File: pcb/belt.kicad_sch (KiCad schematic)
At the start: 2 parts, among them U1 Raspberry-Pi-Pico, U2 Barometer-KP212K1409XTMA1

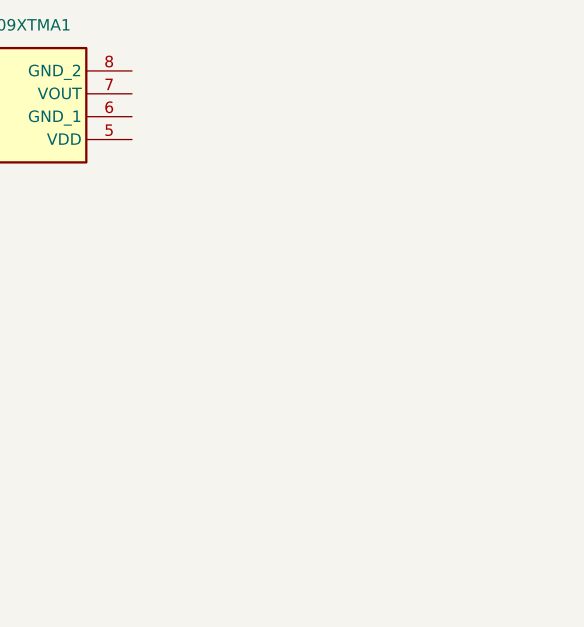
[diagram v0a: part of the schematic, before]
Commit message: added thermometer
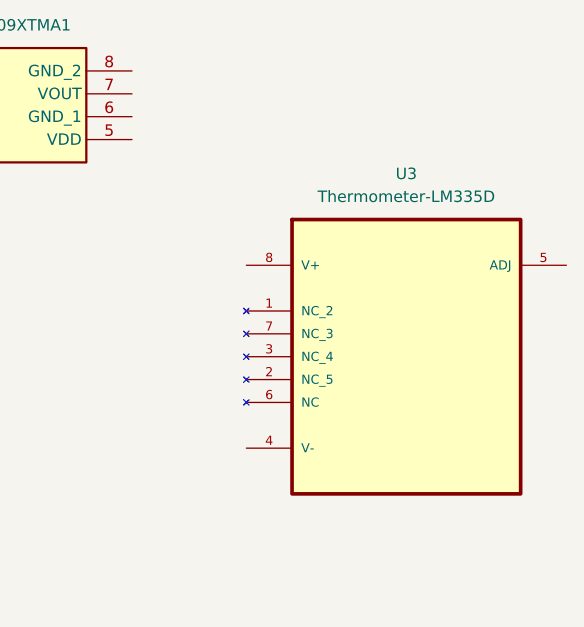
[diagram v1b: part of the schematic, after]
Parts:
- added U3: Thermometer-LM335D, BeltFootprints:Thermometer-LM335D, symbol Thermometer-LM335D:Thermometer-LM335D
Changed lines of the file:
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@@
   (title_block
     (title "Basic Electronics Learning Toolkit")
-    (date "2023-12-25")
+    (date "2023-12-26")
     (rev "0.1")
     (company "Rice Eclipse")
@@
         )
       )
+    )
+  )
+  (symbol (lib_id "Thermometer-LM335D:Thermometer-LM335D") (at 177.8 93.98 0) (unit 1)
+    (in_bom yes) (on_board yes) (dnp no) (fields_autoplaced)
+    (property "Reference" "U3" (at 177.8 73.66 0)
+      (effects (font (size 1.27 1.27)))
+    )
+    (property "Value" "Thermometer-LM335D" (at 177.8 76.2 0)
+      (effects (font (size 1.27 1.27)))
+    )
+    (property "Footprint" "BeltFootprints:Thermometer-LM335D" (at 177.8 116.84 0) (show_name)
+      (effects (font (size 1.27 1.27)) hide)
+    )
+    (property "Datasheet" "https://www.st.com/content/ccc/resource/technical/document/datasheet/04/fa/9d/16/39/87/44/8d/CD00000459.pdf/files/CD00000459.pdf/jcr:content/translations/en.CD00000459.pdf" (at 177.8 119.38 0) (show_name)
+      (effects (font (size 1.27 1.27)) hide)
+    )
+    (property "Manufacturer" "STMicroelectronics" (at 177.8 121.92 0) (show_name)
+      (effects (font (size 1.27 1.27)) hide)
+    )
+    (property "Part Number" "LM335D" (at 177.8 124.46 0) (show_name)
+      (effects (font (size 1.27 1.27)) hide)
+    )
+    (pin "1")
+    (pin "2")
+    (pin "3")
+    (pin "4")
+    (pin "5")
+    (pin "6")
+    (pin "7")
+    (pin "8")
+    (instances
+      (project "belt"
+        (path "/33e5c18d-f516-4ab7-aaea-c68685305111"
+          (reference "U3") (unit 1)
+        )
+      )

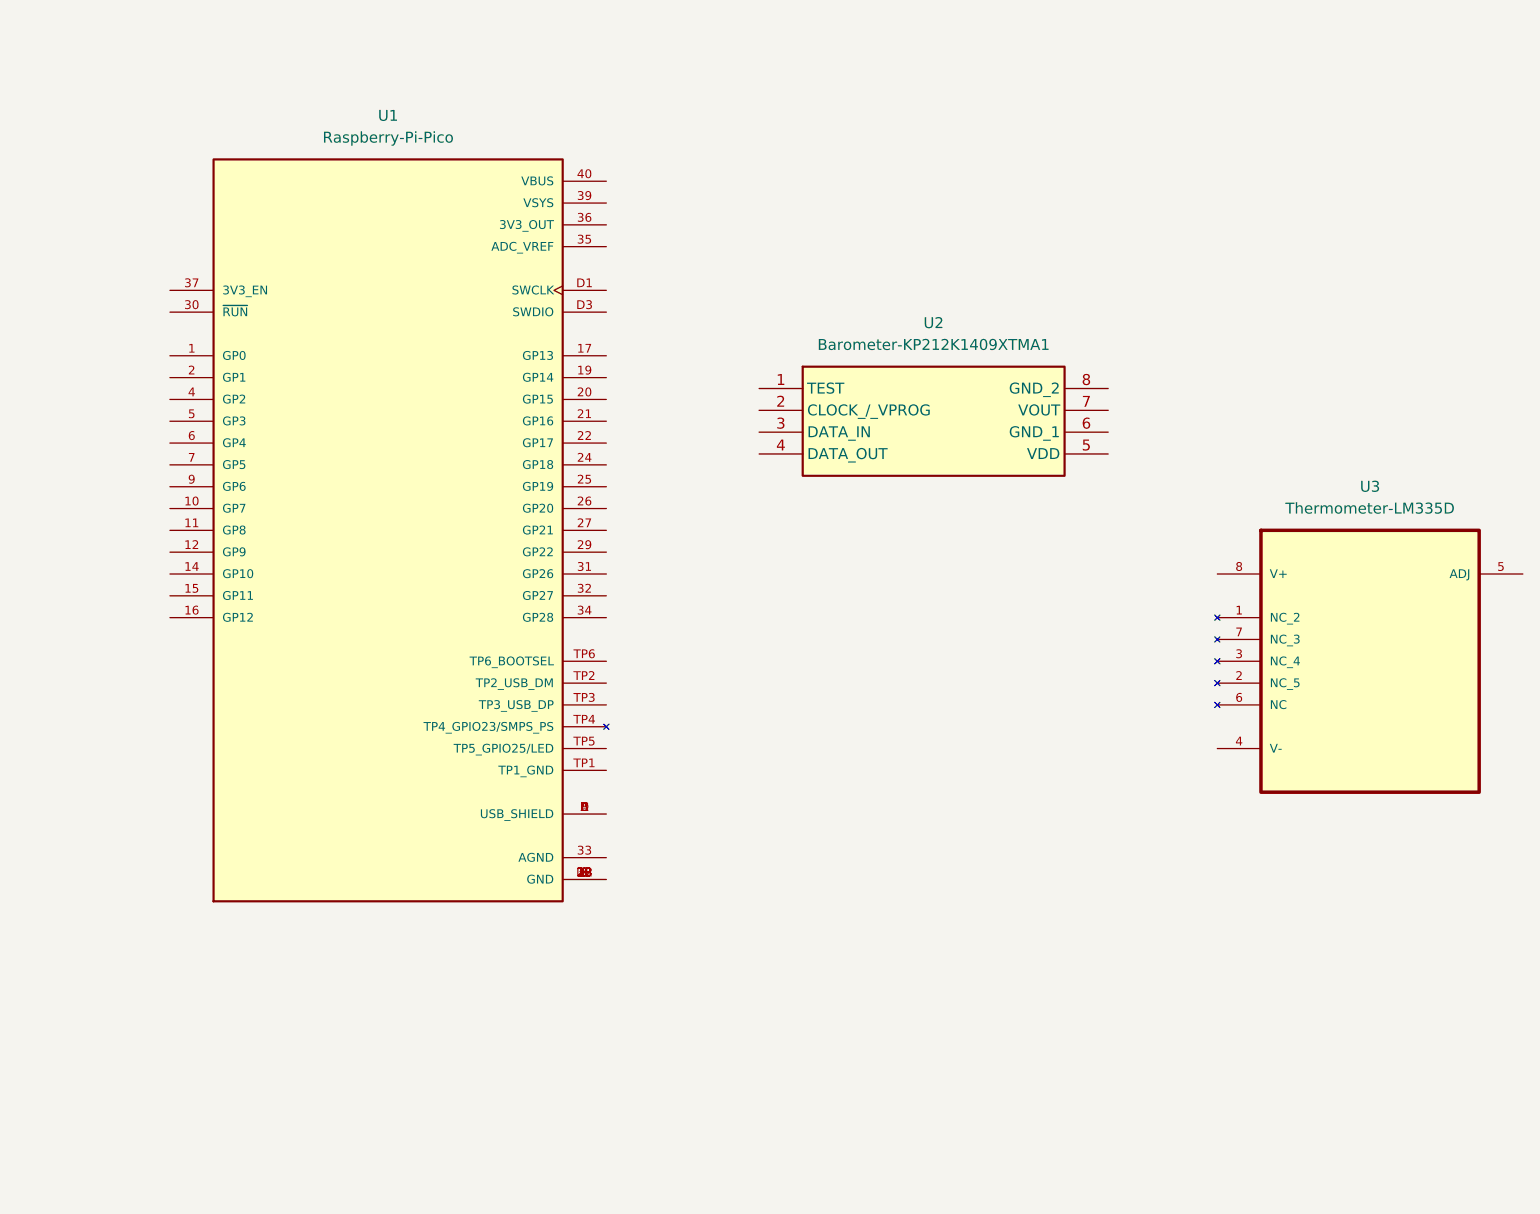
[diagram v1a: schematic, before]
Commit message: wired things up
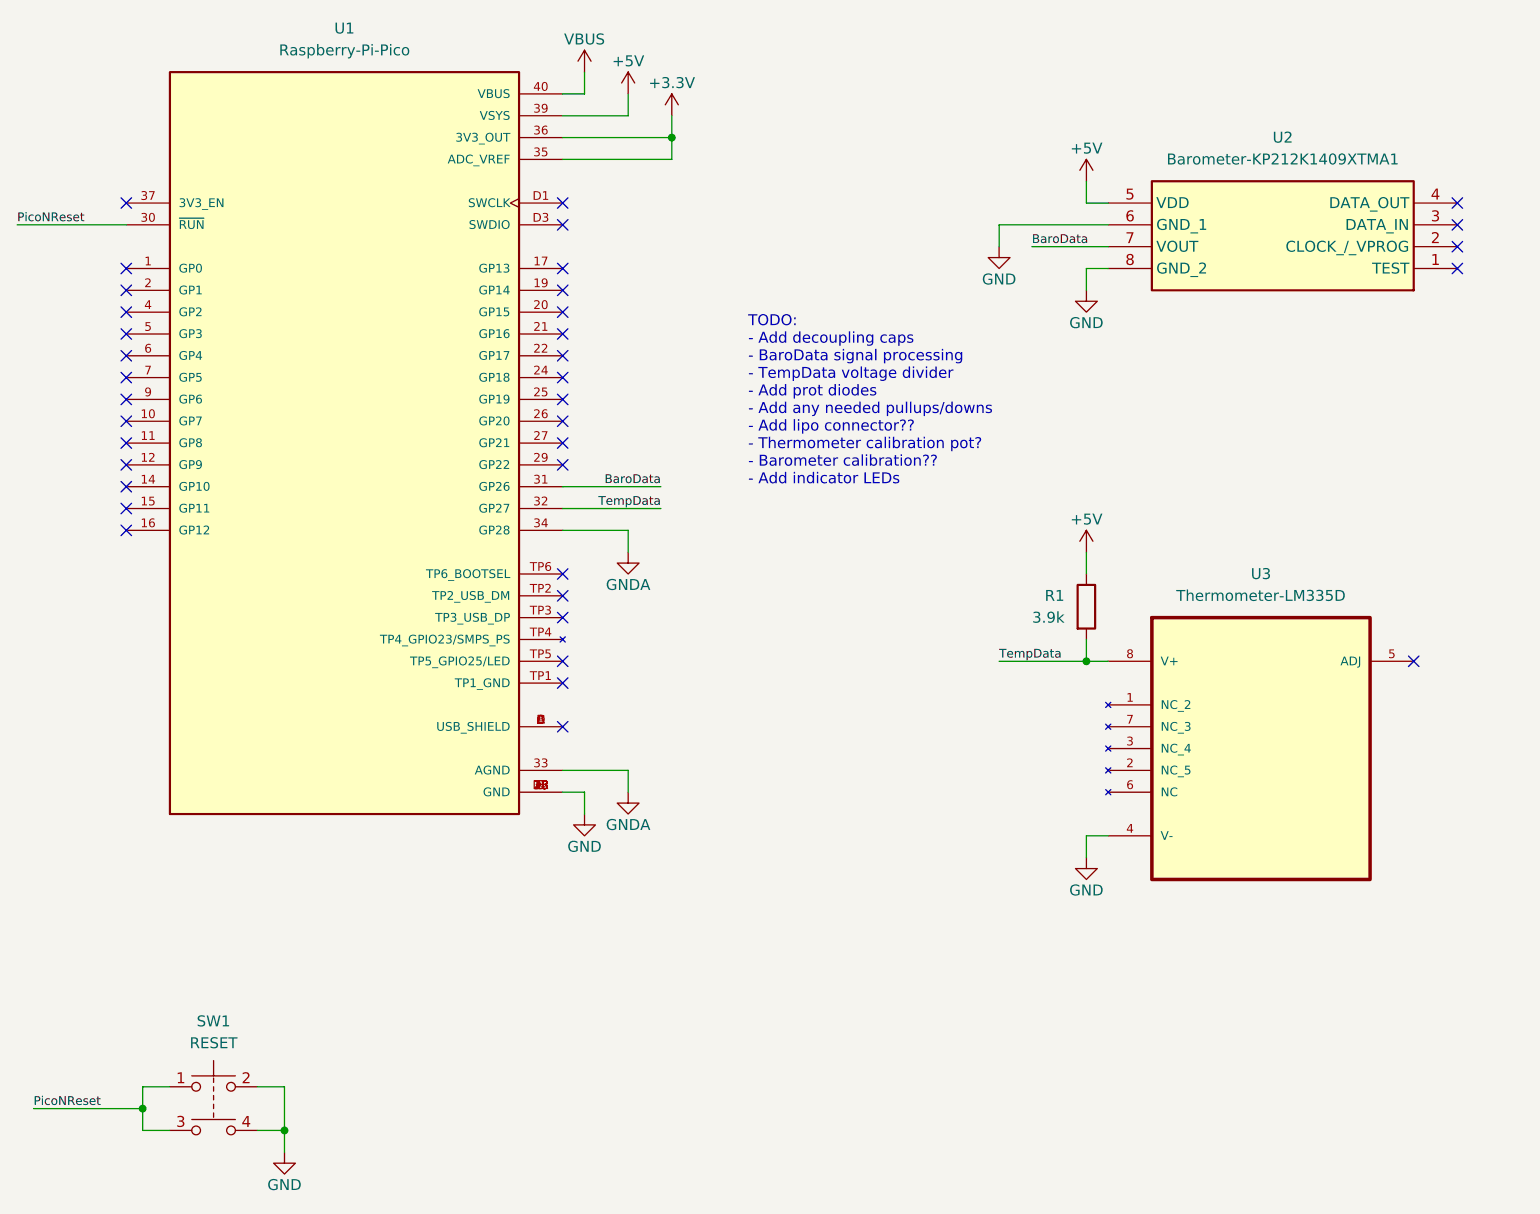
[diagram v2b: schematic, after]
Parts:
- added R1: 3.9k, symbol Device:R
- added SW1: RESET, symbol Switch:SW_Push_Dual
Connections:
- net +5V: now reaches U2.5 (VDD)
- net +5V: now also U1.39 (VSYS), R1.1
- net GND: now reaches U2.6 (GND_1)
- net GND: now also U1.13 (GND), U1.18 (GND), U1.23 (GND), U1.28 (GND), U1.3 (GND), U1.38 (GND), U1.8 (GND), U1.D2 (GND), U2.8 (GND_2), U3.4 (V-), SW1.2, SW1.4
- net BaroData: now reaches U2.7 (VOUT)
- net BaroData: now also U1.31 (GP26)
- net PicoNReset: now reaches U1.30 (~{RUN})
- net PicoNReset: now also SW1.1, SW1.3
- net TempData: now reaches U1.32 (GP27)
- net TempData: now also U3.8 (V+), R1.2
- net GNDA: now reaches U1.33 (AGND)
- net GNDA: now also U1.34 (GP28)
- net +3.3V: now reaches U1.35 (ADC_VREF)
- net +3.3V: now also U1.36 (3V3_OUT)
- net VBUS: now reaches U1.40 (VBUS)
- no-connect marks 0 -> 37
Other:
- note added: "TODO: - Add decoupling caps - BaroData signal processing - TempData voltage divider - Add prot diodes - Add any needed pullups/downs - Add lipo connector?? - Thermometer calibration pot? - Barometer calibration?? - Add indicator LEDs"
- moved on the sheet: U1, U2, U3
